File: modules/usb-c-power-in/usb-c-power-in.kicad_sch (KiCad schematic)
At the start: 2 parts, among them J1 Conn_01x02

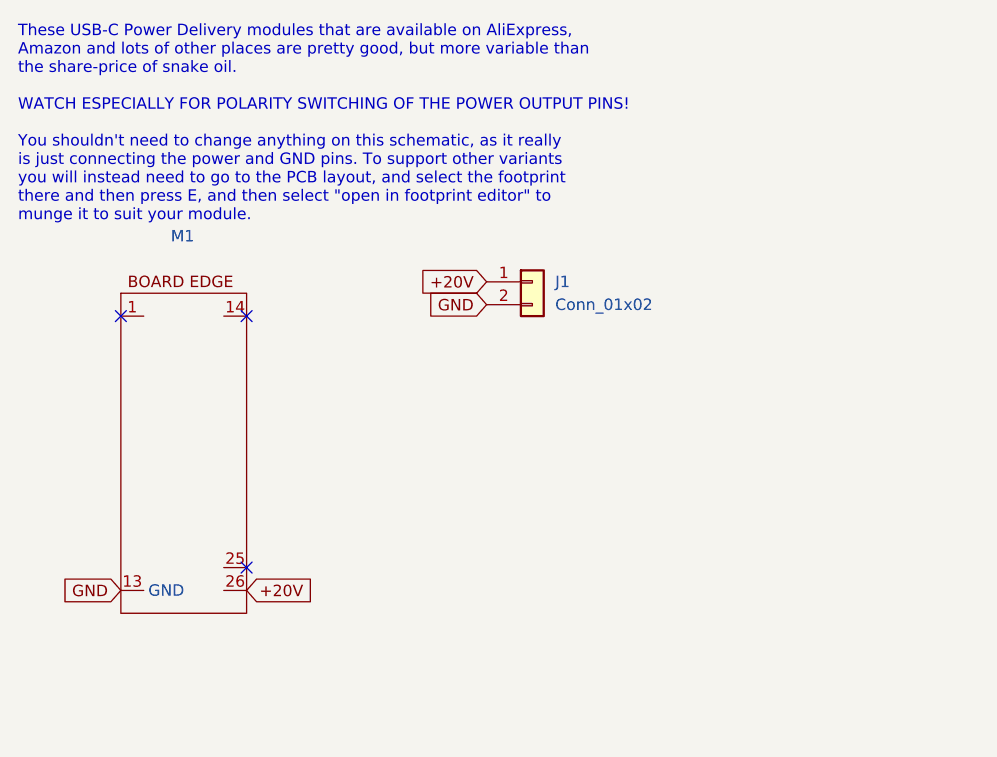
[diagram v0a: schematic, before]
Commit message: Updating all modules
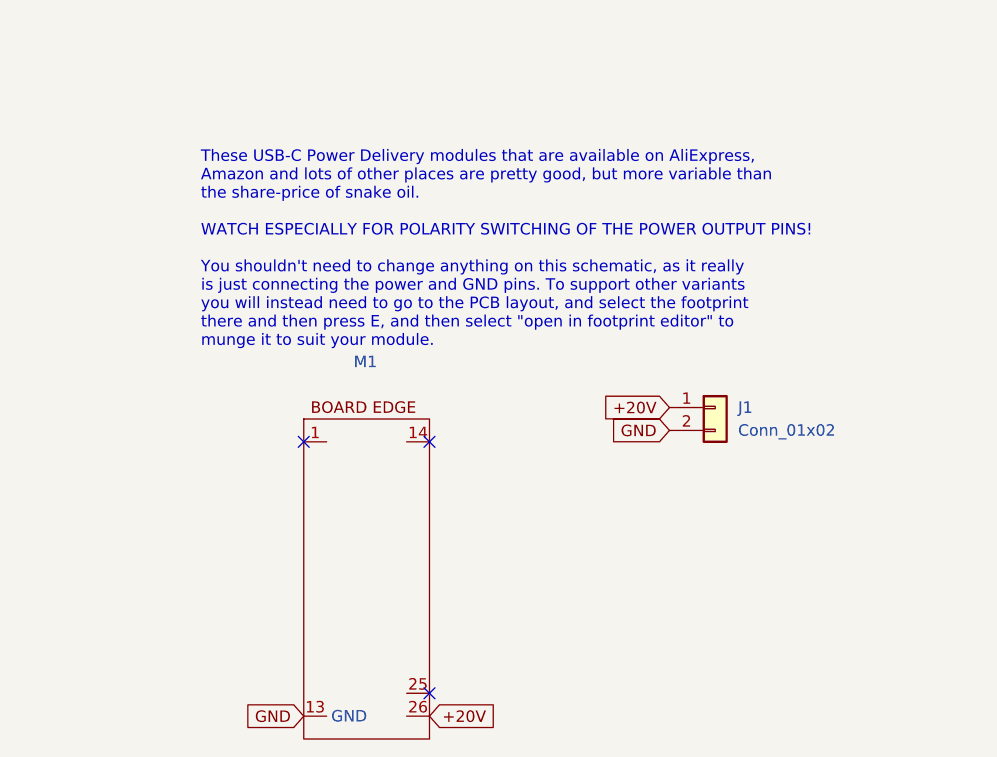
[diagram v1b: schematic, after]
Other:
- moved on the sheet: J1, M1
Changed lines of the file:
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@@
 	(text "These USB-C Power Delivery modules that are available on AliExpress, \nAmazon and lots of other places are pretty good, but more variable than\nthe share-price of snake oil.\n\nWATCH ESPECIALLY FOR POLARITY SWITCHING OF THE POWER OUTPUT PINS!\n\nYou shouldn't need to change anything on this schematic, as it really\nis just connecting the power and GND pins. To support other variants\nyou will instead need to go to the PCB layout, and select the footprint\nthere and then press E, and then select \"open in footprint editor\" to\nmunge it to suit your module."
 		(exclude_from_sim no)
-		(at 29.21 34.544 0)
+		(at 49.53 48.514 0)
 		(effects
 			(font
@@
 	)
 	(no_connect
-		(at 54.61 83.82)
+		(at 74.93 97.79)
 	)
 	(no_connect
-		(at 40.64 55.88)
+		(at 60.96 69.85)
 	)
 	(no_connect
-		(at 54.61 55.88)
+		(at 74.93 69.85)
 	)
 	(global_label "GND"
 		(shape input)
-		(at 40.64 86.36 180)
+		(at 60.96 100.33 180)
 		(fields_autoplaced yes)
 		(effects
@@
 		)
 		(property "Intersheetrefs" "${INTERSHEET_REFS}"
-			(at 33.7843 86.36 0)
+			(at 54.1043 100.33 0)
 			(effects
 				(font
@@
 	(global_label "+20V"
 		(shape input)
-		(at 81.28 52.07 180)
+		(at 101.6 66.04 180)
 		(fields_autoplaced yes)
 		(effects
@@
 		)
 		(property "Intersheetrefs" "${INTERSHEET_REFS}"
-			(at 73.2148 52.07 0)
+			(at 93.5348 66.04 0)
 			(effects
 				(font
@@
 	(global_label "GND"
 		(shape input)
-		(at 81.28 54.61 180)
+		(at 101.6 68.58 180)
 		(fields_autoplaced yes)
 		(effects
@@
 		)
 		(property "Intersheetrefs" "${INTERSHEET_REFS}"
-			(at 74.4243 54.61 0)
+			(at 94.7443 68.58 0)
 			(effects
 				(font
@@
 	(global_label "+20V"
 		(shape input)
-		(at 54.61 86.36 0)
+		(at 74.93 100.33 0)
 		(fields_autoplaced yes)
 		(effects
@@
 		)
 		(property "Intersheetrefs" "${INTERSHEET_REFS}"
-			(at 62.6752 86.36 0)
+			(at 82.9952 100.33 0)
 			(effects
 				(font
@@
 	(symbol
 		(lib_id "MegaCastle:MegaCastle2x13-Module-I14.0x28.2-M800C00C-NOCUTOUT-EDGE")
-		(at 46.99 71.12 0)
+		(at 67.31 85.09 0)
 		(unit 1)
 		(exclude_from_sim no)
@@
 		(fields_autoplaced yes)
 		(property "Reference" "M1"
-			(at 47.4938 46.99 0)
+			(at 67.8138 60.96 0)
 			(effects
 				(font
@@
 		)
 		(property "Value" "~"
-			(at 47.4938 49.53 0)
+			(at 67.8138 63.5 0)
 			(effects
 				(font
@@
 		)
 		(property "Footprint" "MegaCastle:MegaCastle2x13-Module-I20.0x28.2-M800C00C-SPAREPAD"
-			(at 46.99 93.98 0)
+			(at 67.31 107.95 0)
 			(effects
 				(font
@@
 		)
 		(property "Datasheet" ""
-			(at 46.99 66.04 0)
+			(at 67.31 80.01 0)
 			(effects
 				(font
@@
 		)
 		(property "Description" "Generated using footprint-gen .. 14 28 5 M800C00C"
-			(at 46.99 71.12 0)
+			(at 67.31 85.09 0)
 			(effects
 				(font
@@
 	(symbol
 		(lib_id "Connector_Generic:Conn_01x02")
-		(at 86.36 52.07 0)
+		(at 106.68 66.04 0)
 		(unit 1)
 		(exclude_from_sim no)
@@
 		(fields_autoplaced yes)
 		(property "Reference" "J1"
-			(at 88.9 52.0699 0)
+			(at 109.22 66.0399 0)
 			(effects
 				(font
@@
 		)
 		(property "Value" "Conn_01x02"
-			(at 88.9 54.6099 0)
+			(at 109.22 68.5799 0)
 			(effects
 				(font
@@
 		)
 		(property "Footprint" "Connector_PinHeader_2.54mm:PinHeader_1x02_P2.54mm_Vertical"
-			(at 86.36 52.07 0)
+			(at 106.68 66.04 0)
 			(effects
 				(font
@@
 		)
 		(property "Datasheet" "~"
-			(at 86.36 52.07 0)
+			(at 106.68 66.04 0)
 			(effects
 				(font
@@
 		)
 		(property "Description" "Generic connector, single row, 01x02, script generated (kicad-library-utils/schlib/autogen/connector/)"
-			(at 86.36 52.07 0)
-			(effects
-				(font
+			(at 106.68 66.04 0)
+			(effects
+				(font
